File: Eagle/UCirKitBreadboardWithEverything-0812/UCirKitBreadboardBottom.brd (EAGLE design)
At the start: 64.8 x 99.4 mm, 900 parts

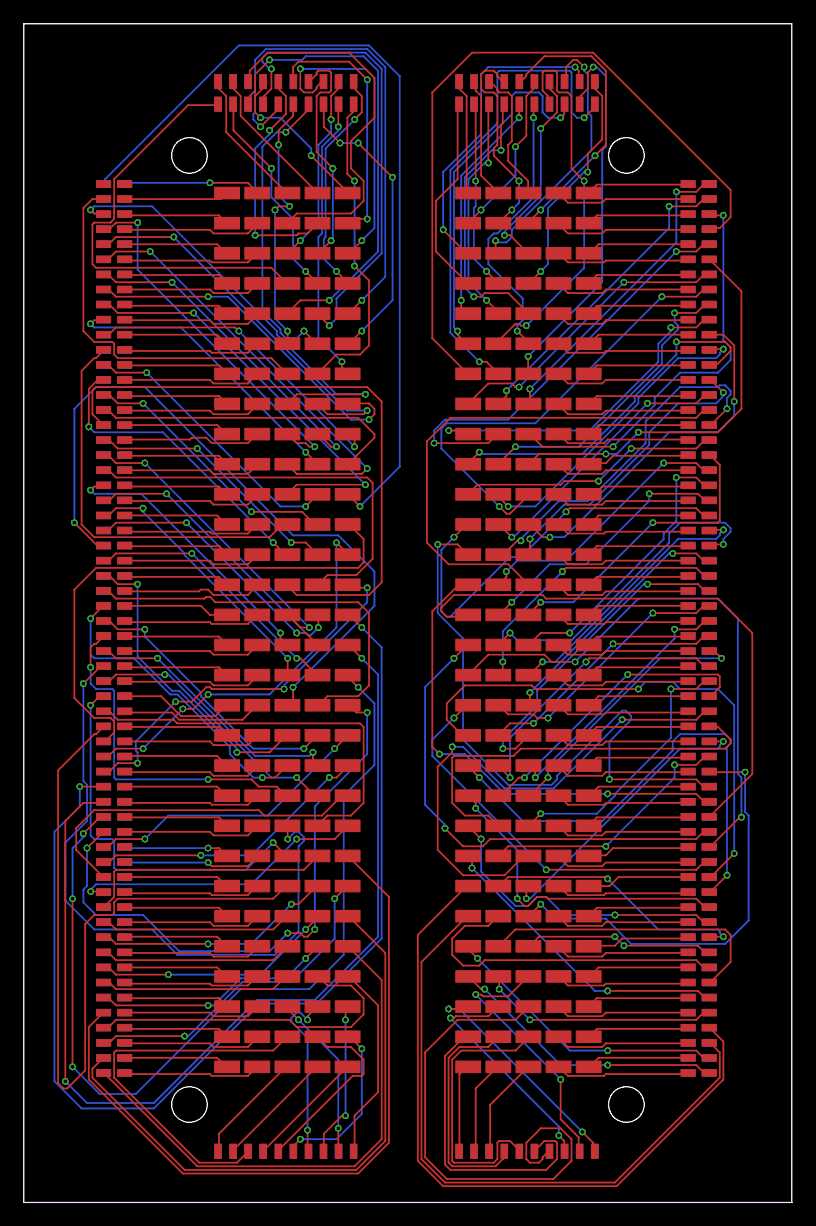
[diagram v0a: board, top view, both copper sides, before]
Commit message: 100% Bottom PCB
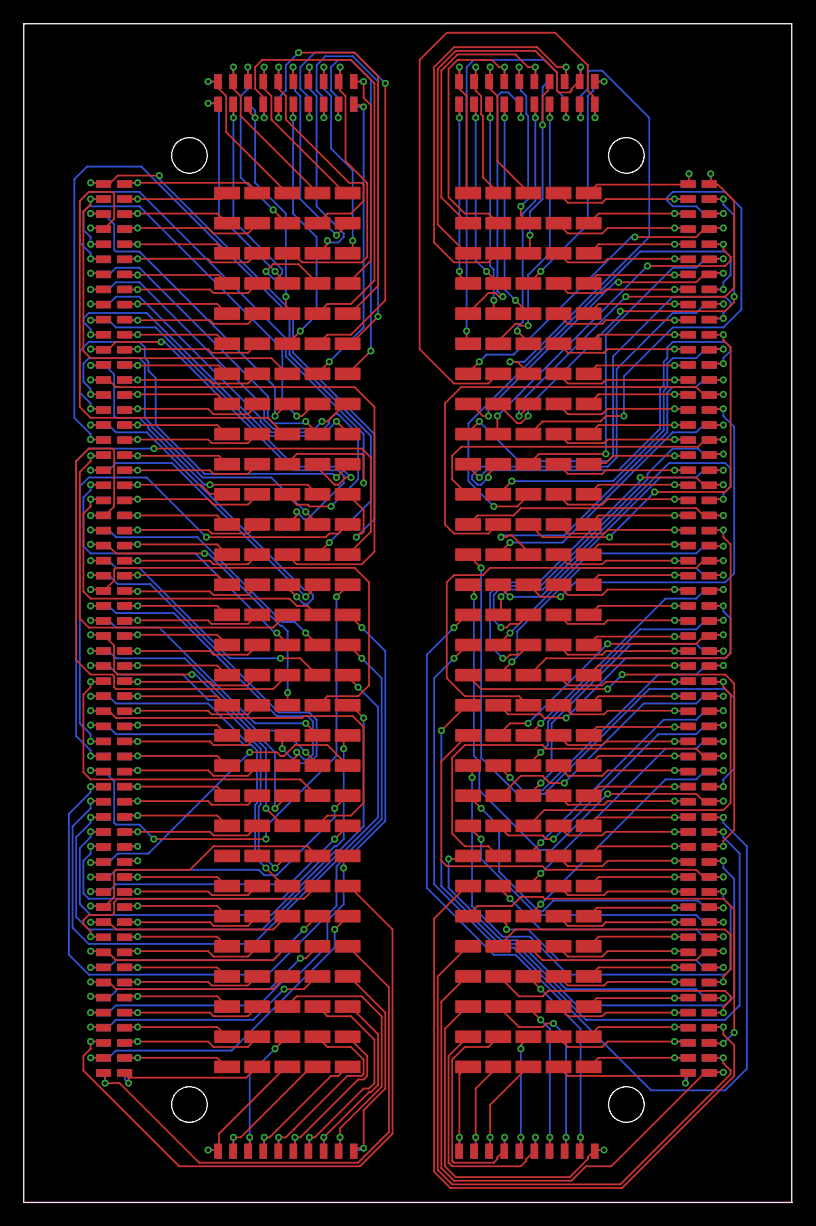
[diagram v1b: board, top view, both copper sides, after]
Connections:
- removed net 0_1439393321: JP661.P$2
- removed net 0_1439394245: JP601.P$2
- removed net N$1000: JP1000.P$2
- removed net N$1001: JP1001.P$2
- removed net N$1002: JP1002.P$2
- removed net N$1003: JP1003.P$2
- removed net N$1004: JP1004.P$2
- removed net N$1007: JP1007.P$2
- removed net N$1008: JP1008.P$2
- removed net N$1009: JP1009.P$2
- removed net N$1010: JP1010.P$2
- removed net N$1011: JP1011.P$2
- removed net N$1012: JP1012.P$2
- removed net N$1013: JP1013.P$2
- removed net N$1014: JP1014.P$2
- removed net N$1015: JP1015.P$2
- removed net N$1016: JP1016.P$2
- removed net N$1017: JP1017.P$2
- removed net N$1018: JP1018.P$2
- removed net N$1019: JP1019.P$2
- removed net N$1020: JP1020.P$2
- removed net N$1021: JP1021.P$2
- removed net N$1022: JP1022.P$2
- removed net N$1023: JP1023.P$2
- removed net N$1024: JP1024.P$2
- removed net N$1025: JP1025.P$2
- removed net N$1026: JP1026.P$2
- removed net N$1027: JP1027.P$2
- removed net N$1028: JP1028.P$2
- removed net N$1029: JP1029.P$2
- removed net N$1030: JP1030.P$2
- removed net N$1031: JP1031.P$2
- removed net N$1032: JP1032.P$2
- removed net N$1033: JP1033.P$2
- removed net N$1034: JP1034.P$2
- removed net N$1035: JP1035.P$2
- removed net N$1036: JP1036.P$2
- removed net N$1037: JP1037.P$2
- removed net N$1038: JP1038.P$2
- removed net N$1039: JP1039.P$2
- removed net N$1040: JP1040.P$2
- removed net N$1041: JP1041.P$2
- removed net N$1042: JP1042.P$2
- removed net N$1043: JP1043.P$2
- removed net N$1044: JP1044.P$2
- removed net N$1045: JP1045.P$2
- removed net N$1046: JP1046.P$2
- removed net N$1047: JP1047.P$2
- removed net N$1048: JP1048.P$2
- removed net N$1049: JP1049.P$2
- removed net N$1050: JP1050.P$2
- removed net N$1051: JP1051.P$2
- removed net N$1052: JP1052.P$2
- removed net N$1053: JP1053.P$2
- removed net N$1054: JP1054.P$2
- removed net N$1055: JP1055.P$2
- removed net N$1056: JP1056.P$2
- removed net N$1057: JP1057.P$2
- removed net N$1058: JP1058.P$2
- removed net N$1059: JP1059.P$2
- removed net N$1060: JP1060.P$2
- removed net N$1061: JP1061.P$2
- removed net N$1062: JP1062.P$2
- removed net N$1063: JP1063.P$2
- removed net N$1064: JP1064.P$2
- removed net N$1065: JP1065.P$2
- removed net N$1066: JP1066.P$2
- removed net N$1067: JP1067.P$2
- removed net N$1068: JP1068.P$2
- removed net N$1069: JP1069.P$2
- removed net N$1070: JP1070.P$2
- removed net N$1071: JP1071.P$2
- removed net N$1072: JP1072.P$2
- removed net N$1073: JP1073.P$2
- removed net N$1074: JP1074.P$2
- removed net N$1075: JP1075.P$2
- removed net N$1076: JP1076.P$2
- removed net N$1077: JP1077.P$2
- removed net N$1078: JP1078.P$2
- removed net N$1079: JP1079.P$2
- removed net N$1080: JP1080.P$2
- removed net N$1081: JP1081.P$2
- removed net N$1082: JP1082.P$2
- removed net N$1083: JP1083.P$2
- removed net N$1084: JP1084.P$2
- removed net N$1085: JP1085.P$2
- removed net N$1086: JP1086.P$2
- removed net N$1087: JP1087.P$2
- removed net N$1088: JP1088.P$2
- removed net N$1089: JP1089.P$2
- removed net N$1090: JP1090.P$2
- removed net N$1091: JP1091.P$2
- removed net N$1092: JP1092.P$2
- removed net N$1093: JP1093.P$2
- removed net N$1094: JP1094.P$2
- removed net N$1095: JP1095.P$2
- removed net N$1096: JP1096.P$2
- removed net N$1097: JP1097.P$2
- removed net N$1098: JP1098.P$2
- removed net N$1099: JP1099.P$2
- removed net N$1100: JP1100.P$2
- removed net N$1101: JP1101.P$2
- removed net N$1102: JP1102.P$2
- removed net N$1103: JP1103.P$2
- removed net N$1104: JP1104.P$2
- removed net N$1105: JP1105.P$2
- removed net N$1106: JP1106.P$2
- removed net N$1107: JP1107.P$2
- removed net N$1108: JP1108.P$2
- removed net N$1109: JP1109.P$2
- removed net N$1110: JP1110.P$2
- removed net N$1111: JP1111.P$2
- removed net N$1112: JP1112.P$2
- removed net N$1113: JP1113.P$2
- removed net N$1114: JP1114.P$2
- removed net N$1115: JP1115.P$2
- removed net N$1116: JP1116.P$2
- removed net N$1117: JP1117.P$2
- removed net N$1118: JP1118.P$2
- removed net N$1119: JP1119.P$2
- removed net N$1120: JP1120.P$2
- removed net N$1121: JP1121.P$2
- removed net N$1122: JP1122.P$2
- removed net N$1123: JP1123.P$2
- removed net N$1124: JP1124.P$2
- removed net N$1125: JP1125.P$2
- removed net N$1126: JP1126.P$2
- removed net N$1127: JP1127.P$2
- removed net N$1128: JP1128.P$2
- removed net N$1129: JP1129.P$2
- removed net N$1130: JP1130.P$2
- removed net N$1131: JP1131.P$2
- removed net N$1132: JP1132.P$2
- removed net N$1133: JP1133.P$2
- removed net N$1134: JP1134.P$2
- removed net N$1135: JP1135.P$2
- removed net N$1136: JP1136.P$2
- removed net N$1137: JP1137.P$2
- removed net N$1138: JP1138.P$2
- removed net N$1139: JP1139.P$2
- removed net N$1140: JP1140.P$2
- removed net N$1141: JP1141.P$2
- removed net N$1142: JP1142.P$2
- removed net N$1143: JP1143.P$2
- removed net N$1144: JP1144.P$2
- removed net N$1145: JP1145.P$2
- removed net N$1146: JP1146.P$2
- removed net N$1147: JP1147.P$2
- removed net N$1148: JP1148.P$2
- removed net N$1149: JP1149.P$2
- removed net N$1150: JP1150.P$2
- removed net N$1151: JP1151.P$2
- removed net N$1152: JP1152.P$2
- removed net N$1153: JP1153.P$2
- removed net N$1154: JP1154.P$2
- removed net N$1155: JP1155.P$2
- removed net N$1156: JP1156.P$2
- removed net N$1157: JP1157.P$2
- removed net N$1158: JP1158.P$2
- removed net N$1159: JP1159.P$2
- removed net N$1160: JP1160.P$2
- removed net N$1161: JP1161.P$2
- removed net N$1162: JP1162.P$2
- removed net N$1163: JP1163.P$2
- removed net N$1164: JP1164.P$2
- removed net N$1165: JP1165.P$2
- removed net N$1166: JP1166.P$2
- removed net N$1167: JP1167.P$2
- removed net N$1168: JP1168.P$2
- removed net N$1169: JP1169.P$2
- removed net N$1170: JP1170.P$2
- removed net N$1171: JP1171.P$2
- removed net N$1172: JP1172.P$2
- removed net N$1173: JP1173.P$2
- removed net N$1174: JP1174.P$2
- removed net N$1175: JP1175.P$2
- removed net N$1176: JP1176.P$2
- removed net N$1177: JP1177.P$2
- removed net N$1178: JP1178.P$2
- removed net N$1179: JP1179.P$2
- removed net N$1180: JP1180.P$2
- removed net N$1181: JP1181.P$2
- removed net N$1182: JP1182.P$2
- removed net N$1183: JP1183.P$2
- removed net N$1184: JP1184.P$2
- removed net N$1185: JP1185.P$2
- removed net N$1186: JP1186.P$2
- removed net N$1187: JP1187.P$2
- removed net N$1188: JP1188.P$2
- removed net N$1189: JP1189.P$2
- removed net N$1190: JP1190.P$2
- removed net N$1191: JP1191.P$2
- removed net N$1192: JP1192.P$2
- removed net N$1193: JP1193.P$2
- removed net N$1194: JP1194.P$2
- removed net N$1195: JP1195.P$2
- removed net N$1196: JP1196.P$2
- removed net N$1197: JP1197.P$2
- removed net N$1198: JP1198.P$2
- removed net N$1199: JP1199.P$2
- removed net N$1200: JP1200.P$2
- removed net N$902: JP902.P$2
- removed net N$903: JP903.P$2
- removed net N$904: JP904.P$2
- removed net N$905: JP905.P$2
- removed net N$906: JP906.P$2
- removed net N$907: JP907.P$2
- removed net N$908: JP908.P$2
- removed net N$909: JP909.P$2
- removed net N$910: JP910.P$2
- removed net N$911: JP911.P$2
- removed net N$912: JP912.P$2
- removed net N$913: JP913.P$2
- removed net N$914: JP914.P$2
- removed net N$915: JP915.P$2
- removed net N$916: JP916.P$2
- removed net N$917: JP917.P$2
- removed net N$918: JP918.P$2
- removed net N$919: JP919.P$2
- removed net N$920: JP920.P$2
- removed net N$921: JP921.P$2
- removed net N$922: JP922.P$2
- removed net N$923: JP923.P$2
- removed net N$924: JP924.P$2
- removed net N$925: JP925.P$2
- removed net N$926: JP926.P$2
- removed net N$927: JP927.P$2
- removed net N$928: JP928.P$2
- removed net N$929: JP929.P$2
- removed net N$930: JP930.P$2
- removed net N$931: JP931.P$2
- removed net N$932: JP932.P$2
- removed net N$933: JP933.P$2
- removed net N$934: JP934.P$2
- removed net N$935: JP935.P$2
- removed net N$936: JP936.P$2
- removed net N$937: JP937.P$2
- removed net N$938: JP938.P$2
- removed net N$939: JP939.P$2
- removed net N$940: JP940.P$2
- removed net N$941: JP941.P$2
- removed net N$942: JP942.P$2
- removed net N$943: JP943.P$2
- removed net N$944: JP944.P$2
- removed net N$945: JP945.P$2
- removed net N$946: JP946.P$2
- removed net N$947: JP947.P$2
- removed net N$948: JP948.P$2
- removed net N$949: JP949.P$2
- removed net N$950: JP950.P$2
- removed net N$951: JP951.P$2
- removed net N$952: JP952.P$2
- removed net N$953: JP953.P$2
- removed net N$954: JP954.P$2
- removed net N$955: JP955.P$2
- removed net N$956: JP956.P$2
- removed net N$957: JP957.P$2
- removed net N$958: JP958.P$2
- removed net N$959: JP959.P$2
- removed net N$960: JP960.P$2
- removed net N$962: JP962.P$2
- removed net N$963: JP963.P$2
- removed net N$964: JP964.P$2
- removed net N$965: JP965.P$2
- removed net N$966: JP966.P$2
- removed net N$967: JP967.P$2
- removed net N$968: JP968.P$2
- removed net N$969: JP969.P$2
- removed net N$970: JP970.P$2
- removed net N$971: JP971.P$2
- removed net N$972: JP972.P$2
- removed net N$973: JP973.P$2
- removed net N$974: JP974.P$2
- removed net N$975: JP975.P$2
- removed net N$976: JP976.P$2
- removed net N$977: JP977.P$2
- removed net N$978: JP978.P$2
- removed net N$979: JP979.P$2
- removed net N$980: JP980.P$2
- removed net N$981: JP981.P$2
- removed net N$982: JP982.P$2
- removed net N$983: JP983.P$2
- removed net N$984: JP984.P$2
- removed net N$985: JP985.P$2
- removed net N$986: JP986.P$2
- removed net N$987: JP987.P$2
- removed net N$988: JP988.P$2
- removed net N$989: JP989.P$2
- removed net N$990: JP990.P$2
- removed net N$991: JP991.P$2
- removed net N$992: JP992.P$2
- removed net N$993: JP993.P$2
- removed net N$994: JP994.P$2
- removed net N$995: JP995.P$2
- removed net N$996: JP996.P$2
- removed net N$997: JP997.P$2
- removed net N$998: JP998.P$2
- removed net N$999: JP999.P$2
- net 0_1439393083: now also JP1019.P$2
- net 0_1439393096: now also JP1017.P$2
- net 0_1439393111: now also JP1015.P$2
- net 0_1439393132: now also JP1005.P$2
- net 0_1439393222: now also JP1013.P$2
- net 0_1439393235: now also JP1011.P$2
- net 0_1439393247: now also JP1009.P$2
- net 0_1439393259: now also JP1007.P$2
- net 0_1439393301: now also JP1006.P$2
- net 0_1439393535: now also JP1003.P$2
- net 0_1439393546: now also JP1001.P$2
- net 0_1439393557: now also JP999.P$2
- net 0_1439393568: now also JP997.P$2
- net 0_1439393578: now also JP995.P$2
- net 0_1439393590: now also JP993.P$2
- net 0_1439393601: now also JP991.P$2
- net 0_1439393611: now also JP989.P$2
- net 0_1439393621: now also JP987.P$2
- net 0_1439393632: now also JP985.P$2
- net 0_1439393643: now also JP983.P$2
- net 0_1439393653: now also JP981.P$2
- net 0_1439393662: now also JP979.P$2
- net 0_1439393672: now also JP977.P$2
- net 0_1439393682: now also JP975.P$2
- net 0_1439393692: now also JP973.P$2
- net 0_1439393702: now also JP971.P$2
- net 0_1439393713: now also JP969.P$2
- net 0_1439393723: now also JP967.P$2
- net 0_1439393733: now also JP965.P$2
- net 0_1439393743: now also JP963.P$2
- net 0_1439393751: now also JP962.P$2
- net 0_1439394322: now also JP1141.P$2
- net 0_1439394368: now also JP1021.P$2
- net 0_1439394379: now also JP1023.P$2
- net 0_1439394391: now also JP1025.P$2
- net 0_1439394441: now also JP1027.P$2
- net 0_1439394451: now also JP1029.P$2
- net 0_1439394459: now also JP1031.P$2
- net 0_1439394467: now also JP1033.P$2
- net 0_1439394476: now also JP1035.P$2
- net 0_1439394485: now also JP1037.P$2
- net 0_1439394493: now also JP1039.P$2
- net 0_1439394502: now also JP1041.P$2
- net 0_1439394512: now also JP1043.P$2
- net 0_1439394521: now also JP1045.P$2
- net 0_1439394528: now also JP1047.P$2
- net 0_1439394536: now also JP1049.P$2
- net 0_1439394545: now also JP1051.P$2
- net 0_1439394554: now also JP1053.P$2
- net 0_1439394565: now also JP1055.P$2
- net 0_1439394575: now also JP1057.P$2
- net 0_1439394583: now also JP1059.P$2
- net 0_1439394592: now also JP1061.P$2
- net 0_1439394601: now also JP1063.P$2
- net 0_1439394609: now also JP1065.P$2
- net 0_1439394617: now also JP1067.P$2
- net 0_1439394705: now also JP1069.P$2
- net 0_1439394717: now also JP1071.P$2
- net 0_1439394727: now also JP1073.P$2
- net 0_1439394736: now also JP1075.P$2
- net 0_1439394745: now also JP1077.P$2
- net 0_1439394755: now also JP1079.P$2
- net 0_1439394769: now also JP1181.P$2
- net 0_1439394798: now also JP1161.P$2
- net 0_1439394824: now also JP1191.P$2
- net 0_1439394861: now also JP902.P$2
- net 0_1439394997: now also JP1081.P$2
- net 10_1439394322: now also JP1151.P$2
- net 10_1439394798: now also JP1171.P$2
- net 10_1439394861: now also JP912.P$2
- net 10_1439394997: now also JP1091.P$2
- net 11_1439394322: now also JP1152.P$2
- net 11_1439394798: now also JP1172.P$2
- net 11_1439394861: now also JP913.P$2
- net 11_1439394997: now also JP1092.P$2
- net 12_1439394322: now also JP1153.P$2
- net 12_1439394798: now also JP1173.P$2
- net 12_1439394861: now also JP914.P$2
- net 12_1439394997: now also JP1093.P$2
- net 13_1439394322: now also JP1154.P$2
- net 13_1439394798: now also JP1174.P$2
- net 13_1439394861: now also JP915.P$2
- net 13_1439394997: now also JP1094.P$2
- net 14_1439394322: now also JP1155.P$2
- net 14_1439394798: now also JP1175.P$2
- net 14_1439394861: now also JP916.P$2
- net 14_1439394997: now also JP1095.P$2
- net 15_1439394322: now also JP1156.P$2
- net 15_1439394798: now also JP1176.P$2
- net 15_1439394861: now also JP917.P$2
- net 15_1439394997: now also JP1096.P$2
- net 16_1439394322: now also JP1157.P$2
- net 16_1439394798: now also JP1177.P$2
- net 16_1439394861: now also JP918.P$2
- net 16_1439394997: now also JP1097.P$2
- net 17_1439394322: now also JP1158.P$2
- net 17_1439394798: now also JP1178.P$2
- net 17_1439394861: now also JP919.P$2
- net 17_1439394997: now also JP1098.P$2
- net 18_1439394322: now also JP1159.P$2
- net 18_1439394798: now also JP1179.P$2
- net 18_1439394861: now also JP920.P$2
- net 18_1439394997: now also JP1099.P$2
- net 19_1439394322: now also JP1160.P$2
- net 19_1439394798: now also JP1180.P$2
- net 19_1439394861: now also JP921.P$2
- net 19_1439394997: now also JP1100.P$2
- net 1_1439393083: now also JP1020.P$2
- net 1_1439393096: now also JP1018.P$2
- net 1_1439393111: now also JP1016.P$2
- net 1_1439393222: now also JP1014.P$2
- net 1_1439393235: now also JP1012.P$2
- net 1_1439393247: now also JP1010.P$2
- net 1_1439393259: now also JP1008.P$2
- net 1_1439393535: now also JP1004.P$2
- net 1_1439393546: now also JP1002.P$2
- net 1_1439393557: now also JP1000.P$2
- net 1_1439393568: now also JP998.P$2
- net 1_1439393578: now also JP996.P$2
- net 1_1439393590: now also JP994.P$2
- net 1_1439393601: now also JP992.P$2
- net 1_1439393611: now also JP990.P$2
- net 1_1439393621: now also JP988.P$2
- net 1_1439393632: now also JP986.P$2
- net 1_1439393643: now also JP984.P$2
- net 1_1439393653: now also JP982.P$2
- net 1_1439393662: now also JP980.P$2
- net 1_1439393672: now also JP978.P$2
- net 1_1439393682: now also JP976.P$2
- net 1_1439393692: now also JP974.P$2
- net 1_1439393702: now also JP972.P$2
- net 1_1439393713: now also JP970.P$2
- net 1_1439393723: now also JP968.P$2
- net 1_1439393733: now also JP966.P$2
- net 1_1439393743: now also JP964.P$2
- net 1_1439394322: now also JP1142.P$2
- net 1_1439394368: now also JP1022.P$2
- net 1_1439394379: now also JP1024.P$2
- net 1_1439394391: now also JP1026.P$2
- net 1_1439394441: now also JP1028.P$2
- net 1_1439394451: now also JP1030.P$2
- net 1_1439394459: now also JP1032.P$2
- net 1_1439394467: now also JP1034.P$2
- net 1_1439394476: now also JP1036.P$2
- net 1_1439394485: now also JP1038.P$2
- net 1_1439394493: now also JP1040.P$2
- net 1_1439394502: now also JP1042.P$2
- net 1_1439394512: now also JP1044.P$2
- net 1_1439394521: now also JP1046.P$2
- net 1_1439394528: now also JP1048.P$2
- net 1_1439394536: now also JP1050.P$2
- net 1_1439394545: now also JP1052.P$2
- net 1_1439394554: now also JP1054.P$2
- net 1_1439394565: now also JP1056.P$2
- net 1_1439394575: now also JP1058.P$2
- net 1_1439394583: now also JP1060.P$2
- net 1_1439394592: now also JP1062.P$2
- net 1_1439394601: now also JP1064.P$2
- net 1_1439394609: now also JP1066.P$2
- net 1_1439394617: now also JP1068.P$2
- net 1_1439394705: now also JP1070.P$2
- net 1_1439394717: now also JP1072.P$2
- net 1_1439394727: now also JP1074.P$2
- net 1_1439394736: now also JP1076.P$2
- net 1_1439394745: now also JP1078.P$2
- net 1_1439394755: now also JP1080.P$2
- net 1_1439394769: now also JP1182.P$2
- net 1_1439394798: now also JP1162.P$2
- net 1_1439394824: now also JP1192.P$2
- net 1_1439394861: now also JP903.P$2
- net 1_1439394997: now also JP1082.P$2
- net 20_1439394861: now also JP922.P$2
- net 20_1439394997: now also JP1101.P$2
- net 21_1439394861: now also JP923.P$2
- net 21_1439394997: now also JP1102.P$2
- net 22_1439394861: now also JP924.P$2
- net 22_1439394997: now also JP1103.P$2
- net 23_1439394861: now also JP925.P$2
- net 23_1439394997: now also JP1104.P$2
- net 24_1439394861: now also JP926.P$2
- net 24_1439394997: now also JP1105.P$2
- net 25_1439394861: now also JP927.P$2
- net 25_1439394997: now also JP1106.P$2
- net 26_1439394861: now also JP928.P$2
- net 26_1439394997: now also JP1107.P$2
- net 27_1439394861: now also JP929.P$2
- net 27_1439394997: now also JP1108.P$2
- net 28_1439394861: now also JP930.P$2
- net 28_1439394997: now also JP1109.P$2
- net 29_1439394861: now also JP931.P$2
- net 29_1439394997: now also JP1110.P$2
- net 2_1439394322: now also JP1143.P$2
- net 2_1439394769: now also JP1183.P$2
- net 2_1439394798: now also JP1163.P$2
- net 2_1439394824: now also JP1193.P$2
- net 2_1439394861: now also JP904.P$2
- net 2_1439394997: now also JP1083.P$2
- net 30_1439394861: now also JP932.P$2
- net 30_1439394997: now also JP1111.P$2
- net 31_1439394861: now also JP933.P$2
- net 31_1439394997: now also JP1112.P$2
- net 32_1439394861: now also JP934.P$2
- net 32_1439394997: now also JP1113.P$2
- net 33_1439394861: now also JP935.P$2
- net 33_1439394997: now also JP1114.P$2
- net 34_1439394861: now also JP936.P$2
- net 34_1439394997: now also JP1115.P$2
- net 35_1439394861: now also JP937.P$2
- net 35_1439394997: now also JP1116.P$2
- net 36_1439394861: now also JP938.P$2
- net 36_1439394997: now also JP1117.P$2
- net 37_1439394861: now also JP939.P$2
- net 37_1439394997: now also JP1118.P$2
- net 38_1439394861: now also JP940.P$2
- net 38_1439394997: now also JP1119.P$2
- net 39_1439394861: now also JP941.P$2
- net 39_1439394997: now also JP1120.P$2
- net 3_1439394322: now also JP1144.P$2
- net 3_1439394769: now also JP1184.P$2
- net 3_1439394798: now also JP1164.P$2
- net 3_1439394824: now also JP1194.P$2
- net 3_1439394861: now also JP905.P$2
- net 3_1439394997: now also JP1084.P$2
- net 40_1439394861: now also JP942.P$2
- net 40_1439394997: now also JP1121.P$2
- net 41_1439394861: now also JP943.P$2
- net 41_1439394997: now also JP1122.P$2
- net 42_1439394861: now also JP944.P$2
- net 42_1439394997: now also JP1123.P$2
- net 43_1439394861: now also JP945.P$2
- net 43_1439394997: now also JP1124.P$2
- net 44_1439394861: now also JP946.P$2
- net 44_1439394997: now also JP1125.P$2
- net 45_1439394861: now also JP947.P$2
- net 45_1439394997: now also JP1126.P$2
- net 46_1439394861: now also JP948.P$2
- net 46_1439394997: now also JP1127.P$2
- net 47_1439394861: now also JP949.P$2
- net 47_1439394997: now also JP1128.P$2
- net 48_1439394861: now also JP950.P$2
- net 48_1439394997: now also JP1129.P$2
- net 49_1439394861: now also JP951.P$2
- net 49_1439394997: now also JP1130.P$2
- net 4_1439394322: now also JP1145.P$2
- net 4_1439394769: now also JP1185.P$2
- net 4_1439394798: now also JP1165.P$2
- net 4_1439394824: now also JP1195.P$2
- net 4_1439394861: now also JP906.P$2
- net 4_1439394997: now also JP1085.P$2
- net 50_1439394861: now also JP952.P$2
- net 50_1439394997: now also JP1131.P$2
- net 51_1439394861: now also JP953.P$2
- net 51_1439394997: now also JP1132.P$2
- net 52_1439394861: now also JP954.P$2
- net 52_1439394997: now also JP1133.P$2
- net 53_1439394861: now also JP955.P$2
- net 53_1439394997: now also JP1134.P$2
- net 54_1439394861: now also JP956.P$2
- net 54_1439394997: now also JP1135.P$2
- net 55_1439394861: now also JP957.P$2
- net 55_1439394997: now also JP1136.P$2
- net 56_1439394861: now also JP958.P$2
- net 56_1439394997: now also JP1137.P$2
- net 57_1439394861: now also JP959.P$2
- net 57_1439394997: now also JP1138.P$2
- net 58_1439394861: now also JP960.P$2
- net 58_1439394997: now also JP1139.P$2
- net 59_1439394997: now also JP1140.P$2
- net 5_1439394322: now also JP1146.P$2
- net 5_1439394769: now also JP1186.P$2
- net 5_1439394798: now also JP1166.P$2
- net 5_1439394824: now also JP1196.P$2
- net 5_1439394861: now also JP907.P$2
- net 5_1439394997: now also JP1086.P$2
- net 60_029414: now also JP601.P$2
- net 60_172194: no longer JP1006.P$2
- net 60_189984: no longer JP1005.P$2
- net 60_19999: now also JP661.P$2
- net 6_1439394322: now also JP1147.P$2
- net 6_1439394769: now also JP1187.P$2
- net 6_1439394798: now also JP1167.P$2
- net 6_1439394824: now also JP1197.P$2
- net 6_1439394861: now also JP908.P$2
- net 6_1439394997: now also JP1087.P$2
- net 7_1439394322: now also JP1148.P$2
- net 7_1439394769: now also JP1188.P$2
- net 7_1439394798: now also JP1168.P$2
- net 7_1439394824: now also JP1198.P$2
- net 7_1439394861: now also JP909.P$2
- net 7_1439394997: now also JP1088.P$2
- net 8_1439394322: now also JP1149.P$2
- net 8_1439394769: now also JP1189.P$2
- net 8_1439394798: now also JP1169.P$2
- net 8_1439394824: now also JP1199.P$2
- net 8_1439394861: now also JP910.P$2
- net 8_1439394997: now also JP1089.P$2
- net 9_1439394322: now also JP1150.P$2
- net 9_1439394769: now also JP1190.P$2
- net 9_1439394798: now also JP1170.P$2
- net 9_1439394824: now also JP1200.P$2
- net 9_1439394861: now also JP911.P$2
- net 9_1439394997: now also JP1090.P$2
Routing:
- net 16_1439394861: track 22.0 -> 73.4 mm
- net 35_1439394861: track 66.1 -> 28.9 mm, vias 0 -> 2
- net 57_1439394997: track 47.8 -> 83.7 mm, vias 0 -> 2
- net 3_1439394997: track 60.8 -> 27.9 mm, vias 0 -> 3
- net 23_1439394861: track 59.7 -> 27.1 mm, vias 2 -> 3
- net 45_1439394861: track 28.0 -> 58.1 mm, vias 2 -> 1
- net 43_1439394861: track 61.5 -> 31.7 mm, vias 0 -> 2
- net 57_1439394861: track 32.7 -> 62.2 mm, vias 4 -> 2
- net 6_1439394824: track 43.3 -> 14.1 mm, vias 0 -> 2
- net 56_1439394997: track 41.1 -> 70.0 mm
- net 31_1439394861: track 54.9 -> 26.3 mm
- net 48_1439394997: track 24.5 -> 53.0 mm, vias 2 -> 1
- net 54_1439394997: track 33.2 -> 59.7 mm
- net 21_1439394861: track 22.7 -> 48.4 mm, vias 2 -> 1
- net 54_1439394861: track 84.5 -> 60.4 mm
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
